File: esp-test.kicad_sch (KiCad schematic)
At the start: 9 parts, among them U1 ESP32-S3-WROOM-1

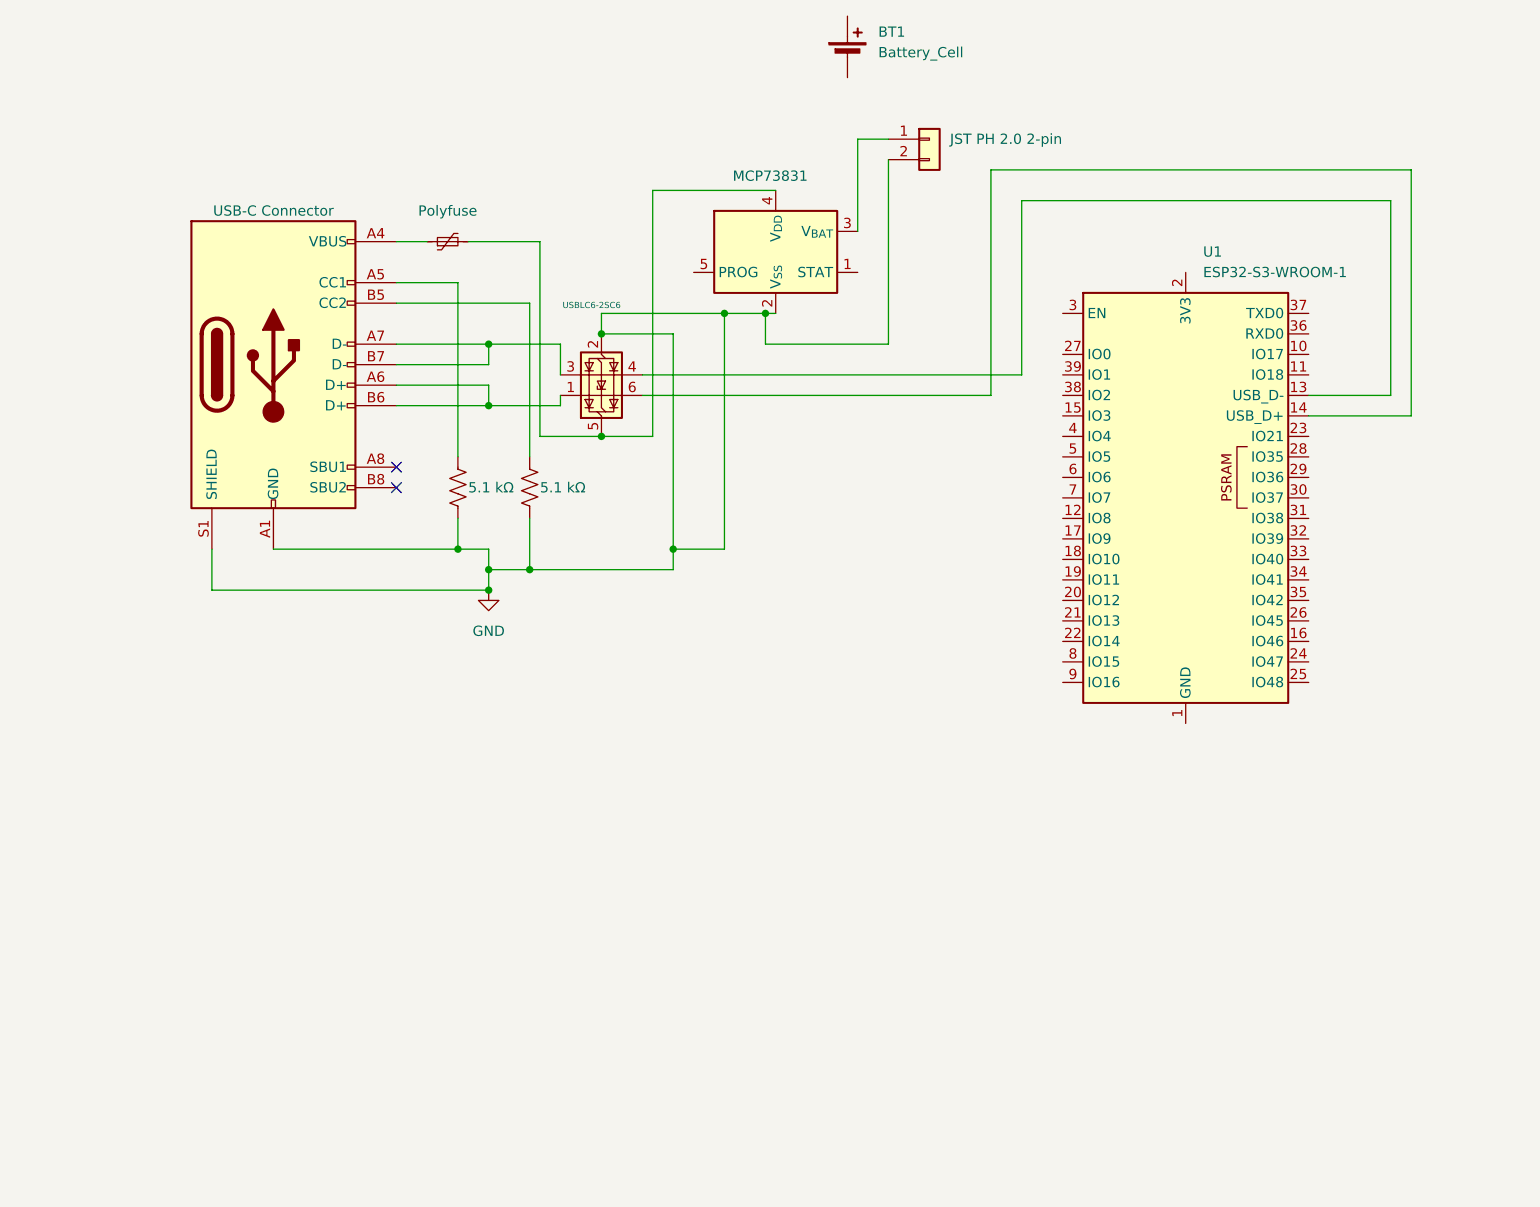
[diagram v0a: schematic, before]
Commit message: work
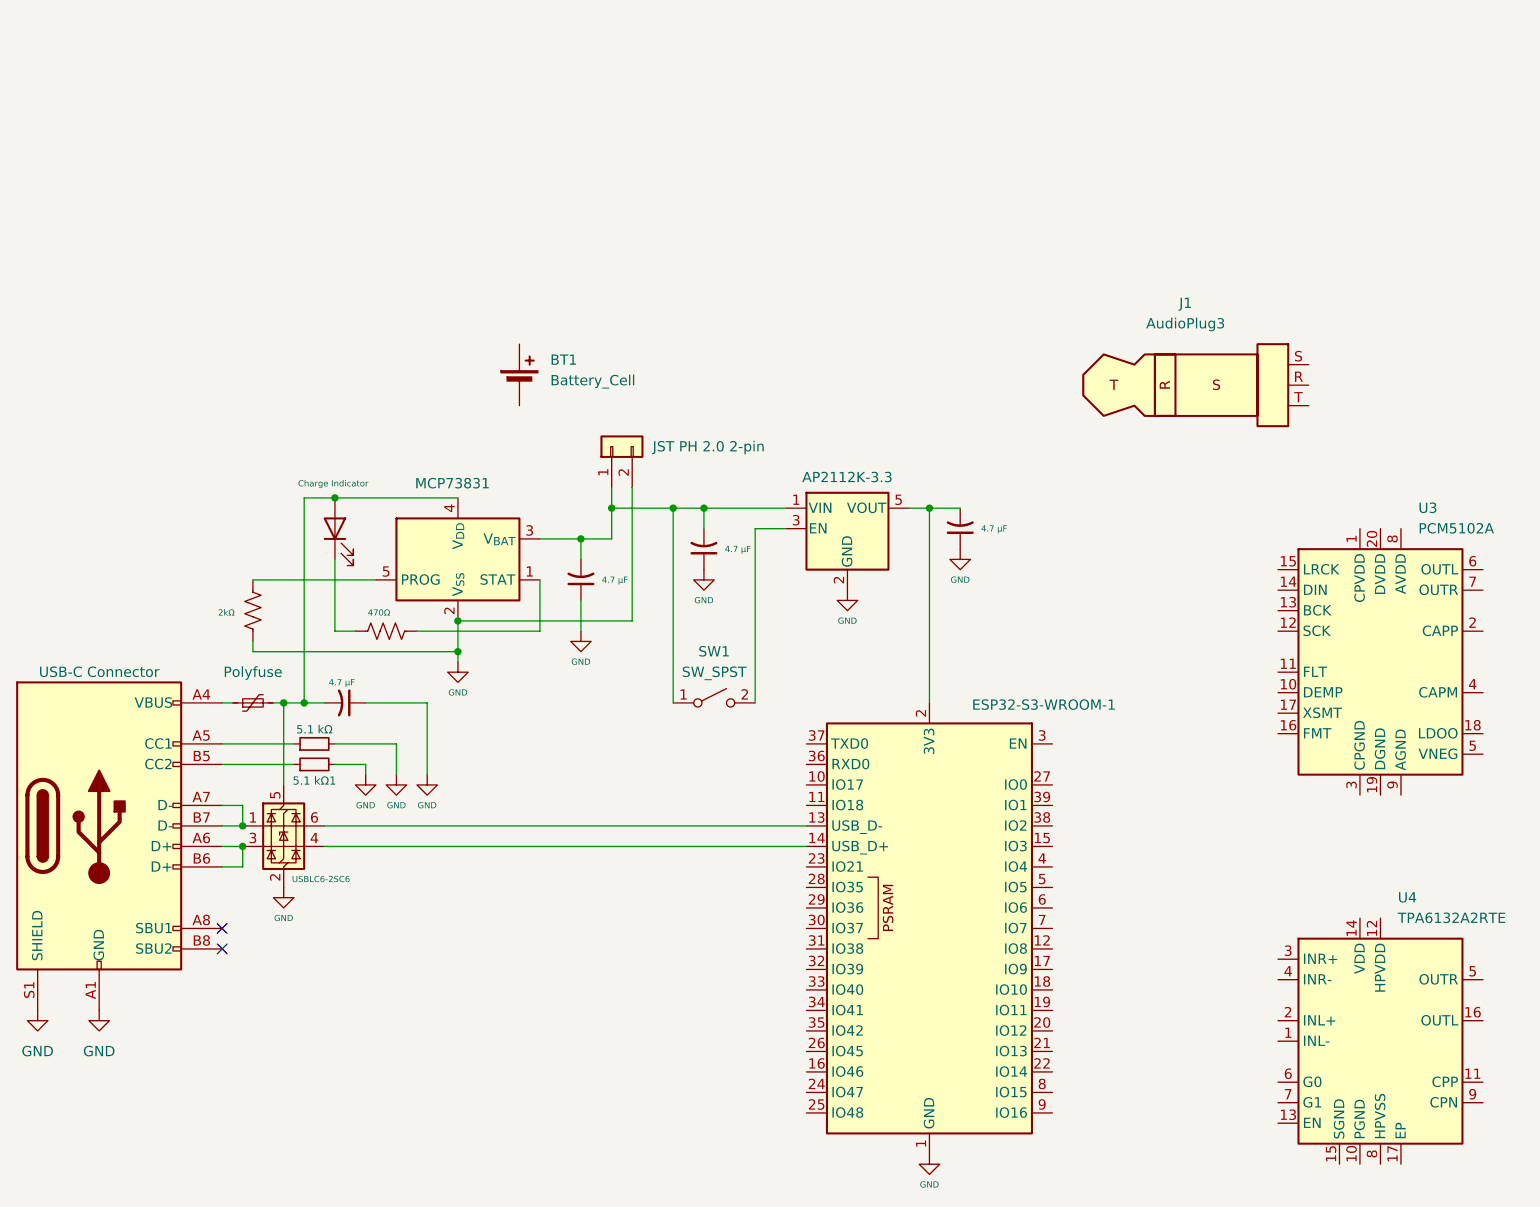
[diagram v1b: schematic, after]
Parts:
- removed 5.1 kΩ: R_US, symbol Device:R_US (x2)
- added 2kΩ, 470Ω: R_US, symbol Device:R_US
- added 5.1 kΩ: R_Small, symbol Device:R_Small
- added 5.1 kΩ1: R_Small, symbol Device:R_Small
- added C1, C2, C3, C4: 4.7 µF, symbol Device:C_Small_US
- added D1: Charge Indicator, symbol Device:LED
- added J1: AudioPlug3, symbol Connector_Audio:AudioPlug3
- added SW1: SW_SPST, symbol Switch:SW_SPST
- added U2: AP2112K-3.3, Package_TO_SOT_SMD:SOT-23-5, symbol Regulator_Linear:AP2112K-3.3
- added U3: PCM5102A, Package_SO:TSSOP-20_4.4x6.5mm_P0.65mm, symbol Audio:PCM5102A
- added U4: TPA6132A2RTE, Package_DFN_QFN:WQFN-16-1EP_3x3mm_P0.5mm_EP1.6x1.6mm_ThermalVias, symbol Amplifier_Audio:TPA6132A2RTE
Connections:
- net GND: now also U1.1 (GND), U1.40 (GND), U1.41 (GND), 2kΩ.2, 5.1 kΩ.2, 5.1 kΩ1.2, C1.1, C2.1, C3.1, C4.1, U2.2 (GND)
- net at USB-C Connector.A5 (CC1): now also 5.1 kΩ.1
- net at USB-C Connector.A6 (D+), USB-C Connector.B6 (D+): now also USBLC6-2SC6.3 (I/O2); no longer USBLC6-2SC6.1 (I/O1)
- net at USB-C Connector.A7 (D-), USB-C Connector.B7 (D-): now also USBLC6-2SC6.1 (I/O1); no longer USBLC6-2SC6.3 (I/O2)
- net at USB-C Connector.B5 (CC2): now also 5.1 kΩ1.1
- net at F1.2, MCP73831.4 (V_{DD}), USBLC6-2SC6.5 (VBUS): now also C1.2, D1.2 (A)
- net at JST PH 2.0 2-pin.1 (Pin_1), MCP73831.3 (V_{BAT}): now also C2.2, C3.2, SW1.1 (A), U2.1 (VIN)
- net at USBLC6-2SC6.4 (I/O2): now also U1.14 (USB_D+); no longer U1.13 (USB_D-)
- net at USBLC6-2SC6.6 (I/O1): now also U1.13 (USB_D-); no longer U1.14 (USB_D+)
- net at MCP73831.1 (STAT): now also 470Ω.1
- net at MCP73831.5 (PROG): now also 2kΩ.1
- net at U1.2 (3V3): now also C4.2, U2.5 (VOUT)
- new net: SW1.2 (B), U2.3 (EN)
- new net: 470Ω.2, D1.1 (K)
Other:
- moved on the sheet: BT1, JST PH 2.0 2-pin, MCP73831, USB-C Connector, USBLC6-2SC6
